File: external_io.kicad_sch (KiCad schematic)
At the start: 19 parts, among them J1 UJ20-C-H-G-SMT-1-P16-TR, J12 Conn_01x03_Socket, J2 Conn_01x02_Socket, J3 Conn_01x03_Socket, J4 Conn_01x04_Socket, J5 Conn_01x03_Socket, J6 Conn_01x03_Socket, U1 USBLC6-2SC6

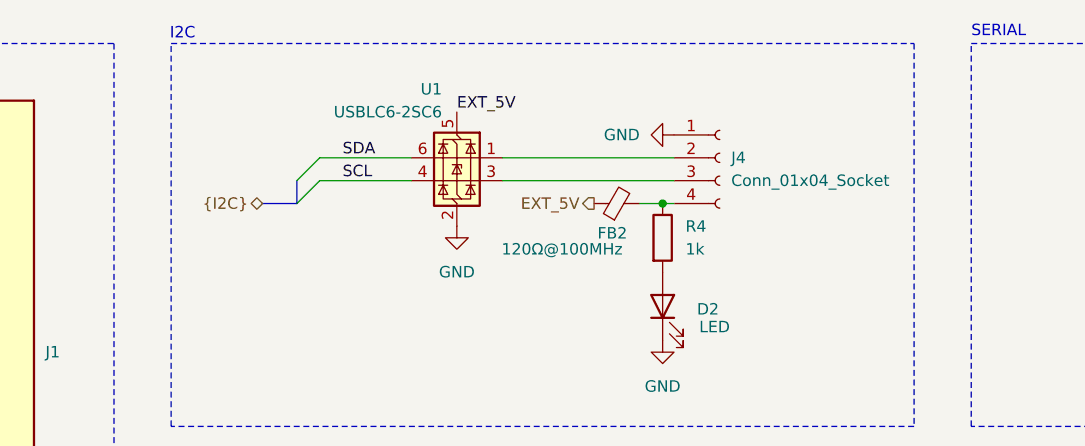
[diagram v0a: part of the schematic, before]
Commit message: Rev3 fixes
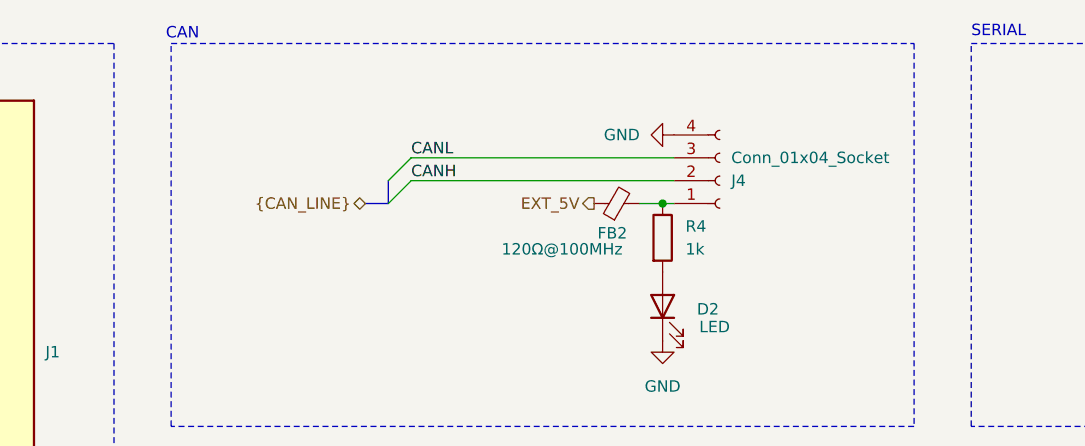
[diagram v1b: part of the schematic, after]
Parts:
- removed U1: USBLC6-2SC6, Package_TO_SOT_SMD:SOT-23-6, symbol Power_Protection:USBLC6-2SC6
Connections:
- net GND: now also J4.4 (Pin_4); no longer J4.1 (Pin_1)
- net at FB2.2, R4.1: now also J4.1 (Pin_1); no longer J4.4 (Pin_4)
- net CANH: now reaches J4.2 (Pin_2)
- net CANL: now reaches J4.3 (Pin_3)
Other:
- note added: "CAN"
- note removed: "I2C"
